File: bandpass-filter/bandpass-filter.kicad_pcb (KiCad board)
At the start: 2 copper layers, 56 x 19 mm, 12 parts, among them J1 Amphenol 10118194-0001LF, J2 Conn_Coaxial, J3 Conn_Coaxial, U1 SKY65015-70LF

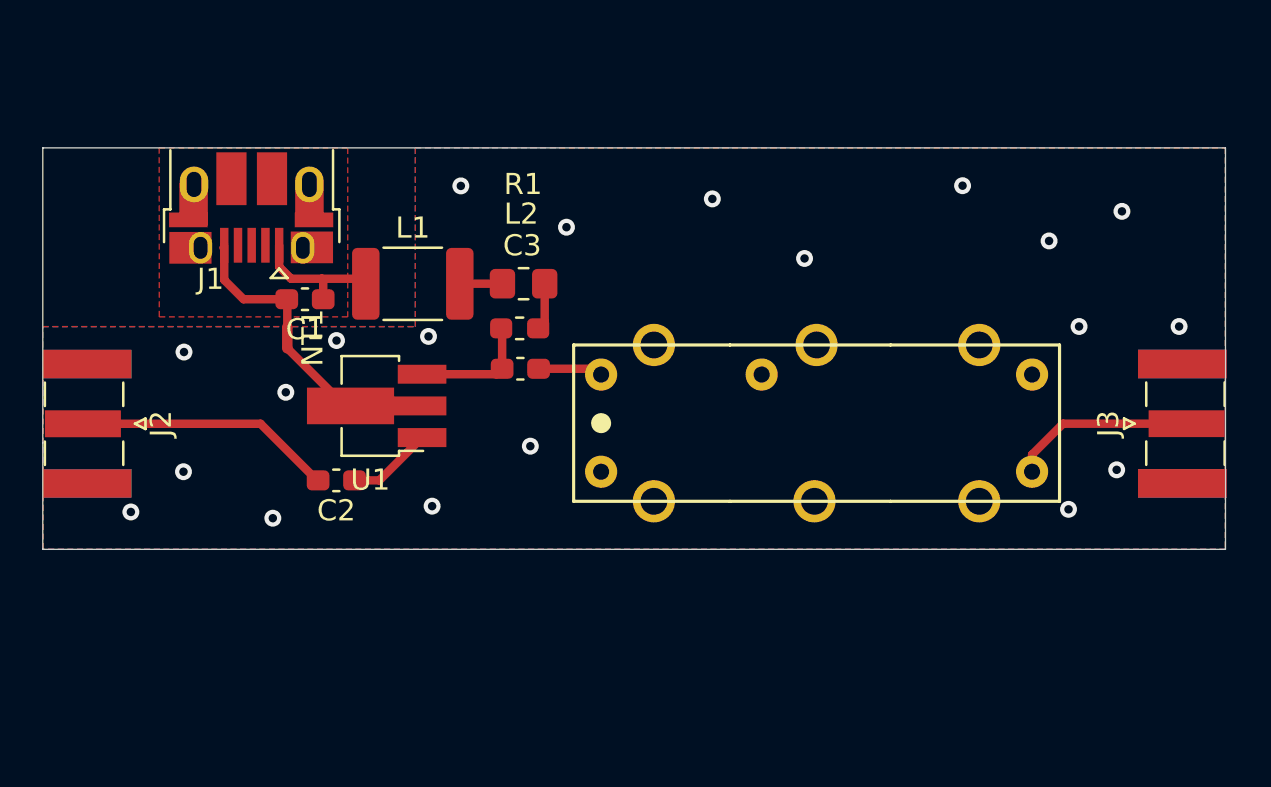
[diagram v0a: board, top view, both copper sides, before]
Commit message: remove todos
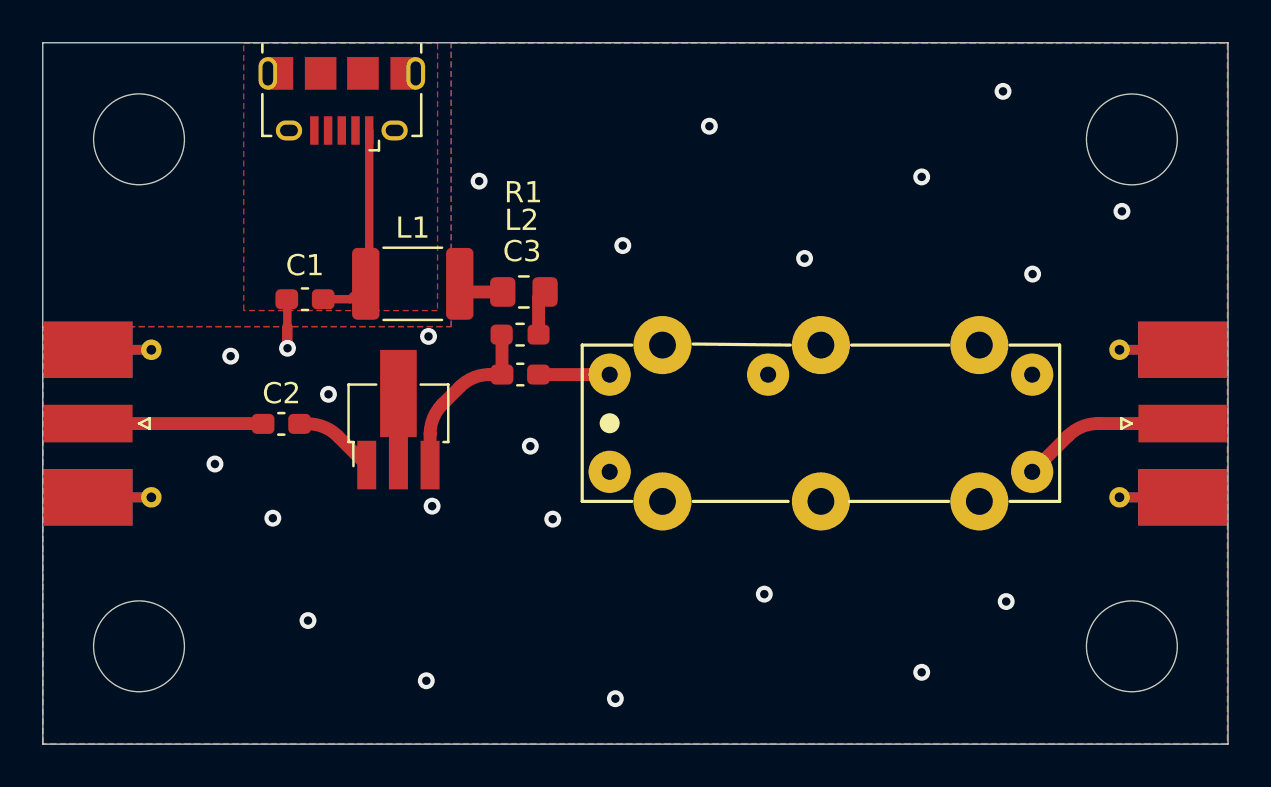
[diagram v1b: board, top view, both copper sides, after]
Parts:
- added H1: MountingHole, MountingHole:MountingHole_4.3mm_M4, F.Cu at (98.2, 40.6)
- added H2: MountingHole, MountingHole:MountingHole_4.3mm_M4, F.Cu at (145.2, 40.6)
- added H3: MountingHole, MountingHole:MountingHole_4.3mm_M4, F.Cu at (98.2, 64.6)
- added H4: MountingHole, MountingHole:MountingHole_4.3mm_M4, F.Cu at (145.2, 64.6)
- J1: footprint Connector_USB:USB_Micro-B_Amphenol_10103594-0001LF_Horizontal -> Connector_USB:USB_Micro-B_Amphenol_10118194_Horizontal
- J2, J3: footprint Connector_Coaxial:SMA_Samtec_SMA-J-P-X-ST-EM1_EdgeMount -> Connector_Coaxial:SMA_Molex_73251-2120_EdgeMount_Horizontal
- moved J1 6.64 mm to (107.8, 38.8)
- moved C2 3.73 mm to (105.0, 54.0)
- moved F1 2.86 mm to (138.0, 50.3)
- moved U1 1.22 mm to (110.5, 53.8), turned to 90 degrees
- moved R1 0.39 mm to (116.5, 47.8)
- moved L2 0.30 mm to (116.3, 49.8)
- moved C3 0.28 mm to (116.3, 51.7)
- moved J2 0.06 mm to (95.8, 54.0), turned to 180 degrees
- turned J3 to 0 degrees
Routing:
- net GNDA: track 7.42 -> 0.01 mm, vias 20 -> 23
- net GNDD: track 8.02 -> 1.30 mm
- net Net-(C2-Pad2): track 12.2 -> 8.28 mm
- net +5VD: track 6.88 -> 9.65 mm
- net Net-(C3-Pad2): track 5.83 -> 8.23 mm
- net Net-(F1-Pad5): track 8.73 -> 7.97 mm
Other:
- board size 56 x 19 mm -> 56.1 x 33.2 mm
- net class Default removed
